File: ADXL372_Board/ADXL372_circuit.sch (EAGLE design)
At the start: 11 parts, among them U1 STM32F030C8T6, U2 ADXL345BCCZ, U3 ADXL372BCCZ-RL7

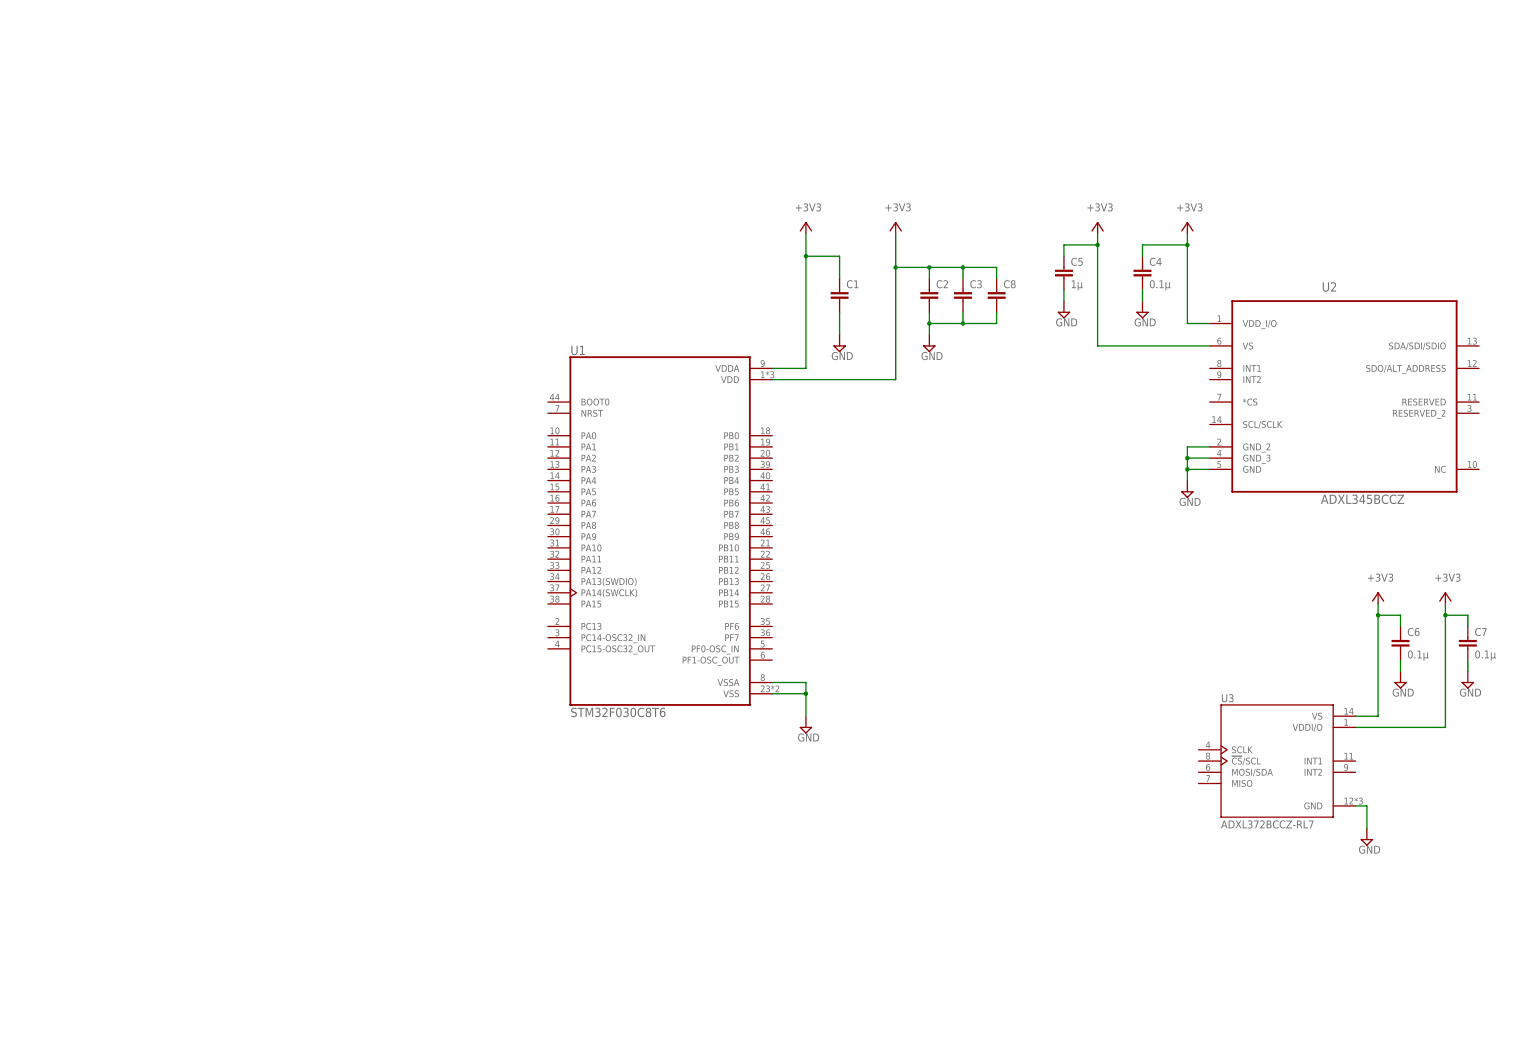
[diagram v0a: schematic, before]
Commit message: Add Parts
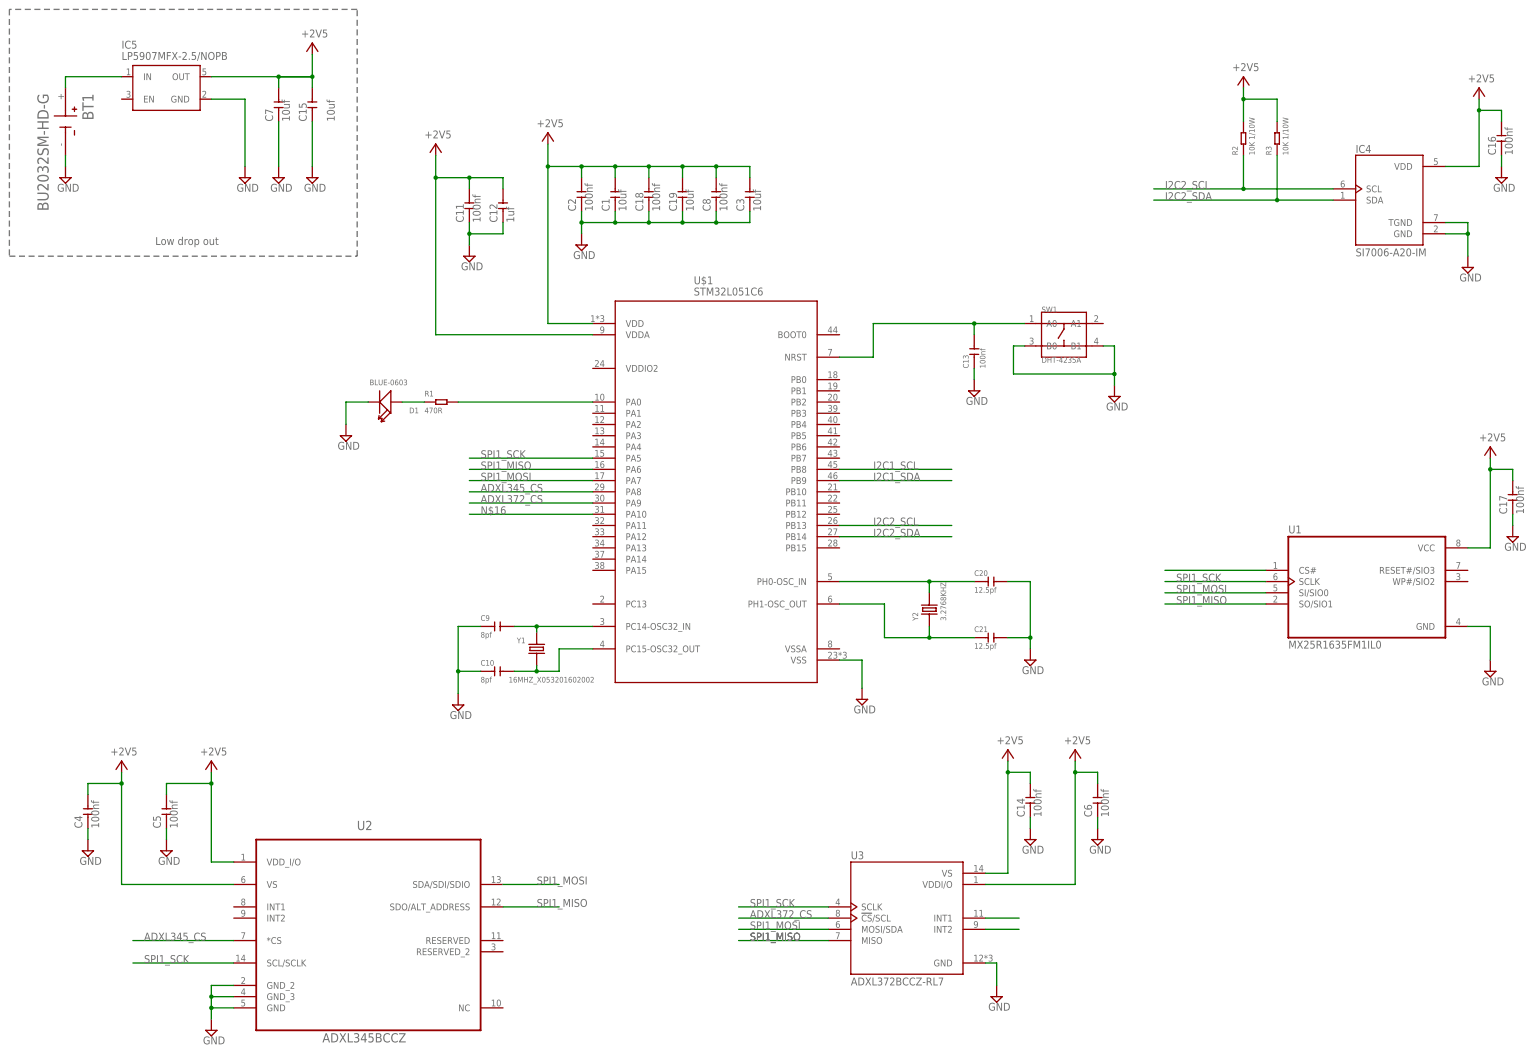
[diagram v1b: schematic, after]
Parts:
- added BT1: BU2032SM-HD-G, BU2032SM-HD-G:BU2032SM-HD-G
- added C10, C9: 8pf, OPL_Capacitor:CERAMIC-10PF-50V-5%-NPO(0603)
- added C11, C13, C14, C16, C17, C18: 100nf, OPL_Capacitor:CERAMIC-100NF-50V-10%-X7R(0603)
- added C12: 1uf, OPL_Capacitor:CERAMIC-1UF-25V-10%-X7R(0805)
- added C15, C19: 10uf, OPL_Capacitor:CERAMIC-10UF-10V-(-20%～+80%)-Y5V(0805)
- added C20, C21: 12.5pf, OPL_Capacitor:CERAMIC-10PF-50V-5%-NPO(0603)
- added D1: BLUE-0603, Seeed-LED:SMD-LED-CLEAR-BLUE(0603)
- added IC4: SI7006-A20-IM, SI7006-A20-IM:SI7006-A20-IM
- added IC5: LP5907MFX-2.5/NOPB, LP5907MFX-2.5_NOPB:LP5907MFX-2.5/NOPB
- added R1: 470R, OPL_Resistor:SMD-RES-470R-5%-1/10W(0603)
- added R2, R3: 10K 1/10W, OPL_Resistor:SMD-RES-10K-5%-1/10W(0603)
- added SW1: DHT-4235A, OPL_Switch:SMD-BUTTON-TOP-DHT-4235A(4P-4.2X3.2MM)
- added U$1: STM32L051C6, stm32l05x6:STM32L051C6
- added Y1: 16MHZ_X053201602002, OPL_Crystal Oscillator:SMD-CRYSTAL-16MHZ-8PF-20PPM-40R(2P-5.0X3.2MM)
- added Y2: 3.2768KHZ, OPL_Crystal Oscillator:SMD-CRYSTAL-32.768KHZ-12.5PF-20PPM-90K(2P-L2.0X1.2MM)
- C1, C3: value (none) -> 10uf; device rcl:C-EUC0603K -> OPL_Capacitor:CERAMIC-10UF-10V-(-20%～+80%)-Y5V(0805)
- C2, C8: value (none) -> 100nf; device rcl:C-EUC0603K -> OPL_Capacitor:CERAMIC-100NF-50V-10%-X7R(0603)
- C4, C6: value 0.1μ -> 100nf; device rcl:C-EUC0603K -> OPL_Capacitor:CERAMIC-100NF-50V-10%-X7R(0603)
- C5: value 1μ -> 100nf; device rcl:C-EUC0603K -> OPL_Capacitor:CERAMIC-100NF-50V-10%-X7R(0603)
- C7: value 0.1μ -> 10uf; device rcl:C-EUC0603K -> OPL_Capacitor:CERAMIC-10UF-10V-(-20%～+80%)-Y5V(0805)
- U1: value STM32F030C8T6 -> MX25R1635FM1IL0; device STM32F030C8T6:STM32F030C8T6 -> MX25R1635FM1IL0:MX25R1635FM1IL0
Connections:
- new net +2V5: C1.2, C11.2, C12.2, C15.2, C18.2, C19.2, C2.2, C3.2, C7.2, C8.2, IC5.OUT, U$1.VDD, U$1.VDDA
- new net ADXL345_CS: U$1.PA8
- new net ADXL372_CS: U$1.PA9
- new net I2C1_SCL: U$1.PB8
- new net I2C1_SDA: U$1.PB9
- new net I2C2_SCL: IC4.SCL, R2.1, U$1.PB13
- new net I2C2_SDA: IC4.SDA, R3.1, U$1.PB14
- new net N$1: C9.2, U$1.PC14-OSC32_IN, Y1.2
- new net N$10: U2.SDA/SDI/SDIO
- new net N$11: U2.SDO/ALT_ADDRESS
- new net N$12: U3.INT1
- new net N$13: U3.INT2
- new net N$14: C20.1, U$1.PH0-OSC_IN, Y2.2
- new net N$15: C21.1, U$1.PH1-OSC_OUT, Y2.1
- new net N$16: U$1.PA10
- new net N$19: R1.2, U$1.PA0
- new net N$2: C10.2, U$1.PC15-OSC32_OUT, Y1.1
- new net N$20: D1.+, R1.1
- new net N$22: BT1.+, IC5.IN
- new net N$24: U1.CS#
- new net N$3: C13.2, SW1.A0, U$1.NRST
- new net N$4: U2.SCL/SCLK
- new net N$5: U3.SCLK
- new net N$6: U3.!CS!/SCL
- new net N$7: U3.MOSI/SDA
- new net N$8: U3.MISO
- new net N$9: U2.*CS
- new net SPI1_MISO: U$1.PA6, U1.SO/SIO1
- new net SPI1_MOSI: U$1.PA7, U1.SI/SIO0
- new net SPI1_SCK: U$1.PA5, U1.SCLK
- net +3V3: now also C14.2, C16.2, C17.2, C4.2, C5.2, C6.2, IC4.VDD, R2.2, R3.2, U1.VCC; no longer C1.1, C2.1, C3.1, C4.1, C5.1, C6.1, C7.1, C8.1, U1.VDD, U1.VDDA
- net GND: now also BT1.-, C1.1, C10.1, C11.1, C12.1, C13.1, C14.1, C15.1, C16.1, C17.1, C18.1, C19.1, C2.1, C20.2, C21.2, C3.1, C4.1, C5.1, C6.1, C7.1, C8.1, C9.1, D1.-, IC4.GND, IC4.TGND, IC5.GND, SW1.B0, SW1.B1, U$1.VSS, U1.GND; no longer C1.2, C2.2, C3.2, C4.2, C5.2, C6.2, C7.2, C8.2, U1.VSS, U1.VSSA
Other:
- note added: "Low drop out"
- moved on the sheet: U2, U3
